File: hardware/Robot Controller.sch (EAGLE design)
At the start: 17 parts

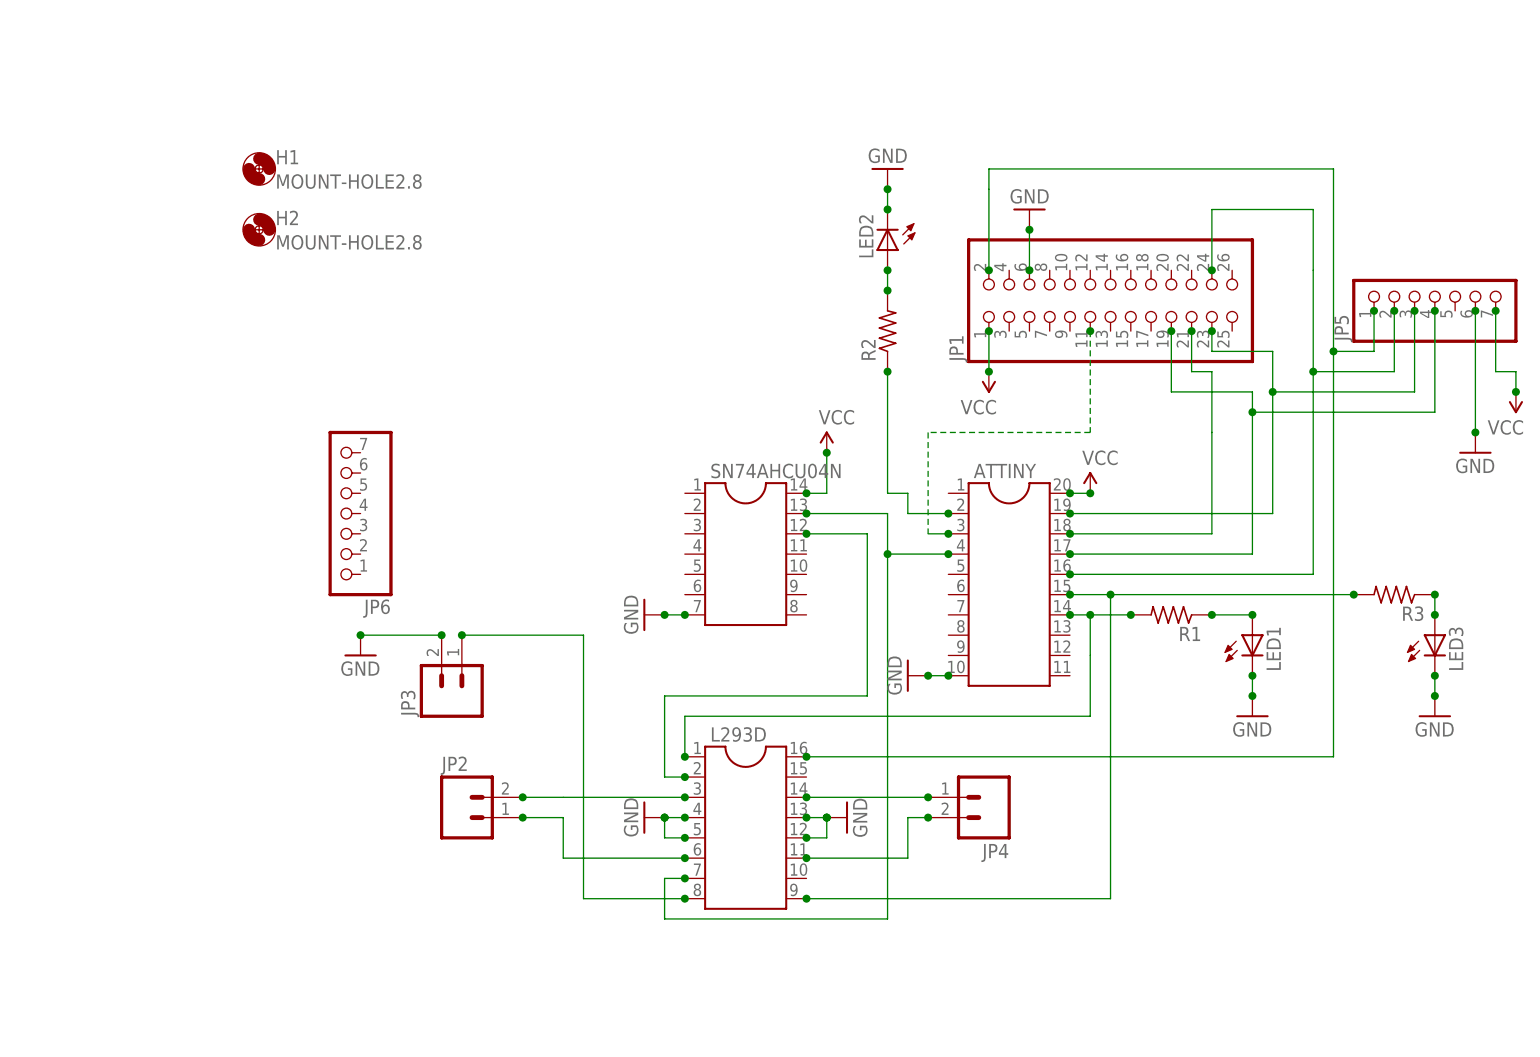
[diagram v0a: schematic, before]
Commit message: WIP dev board
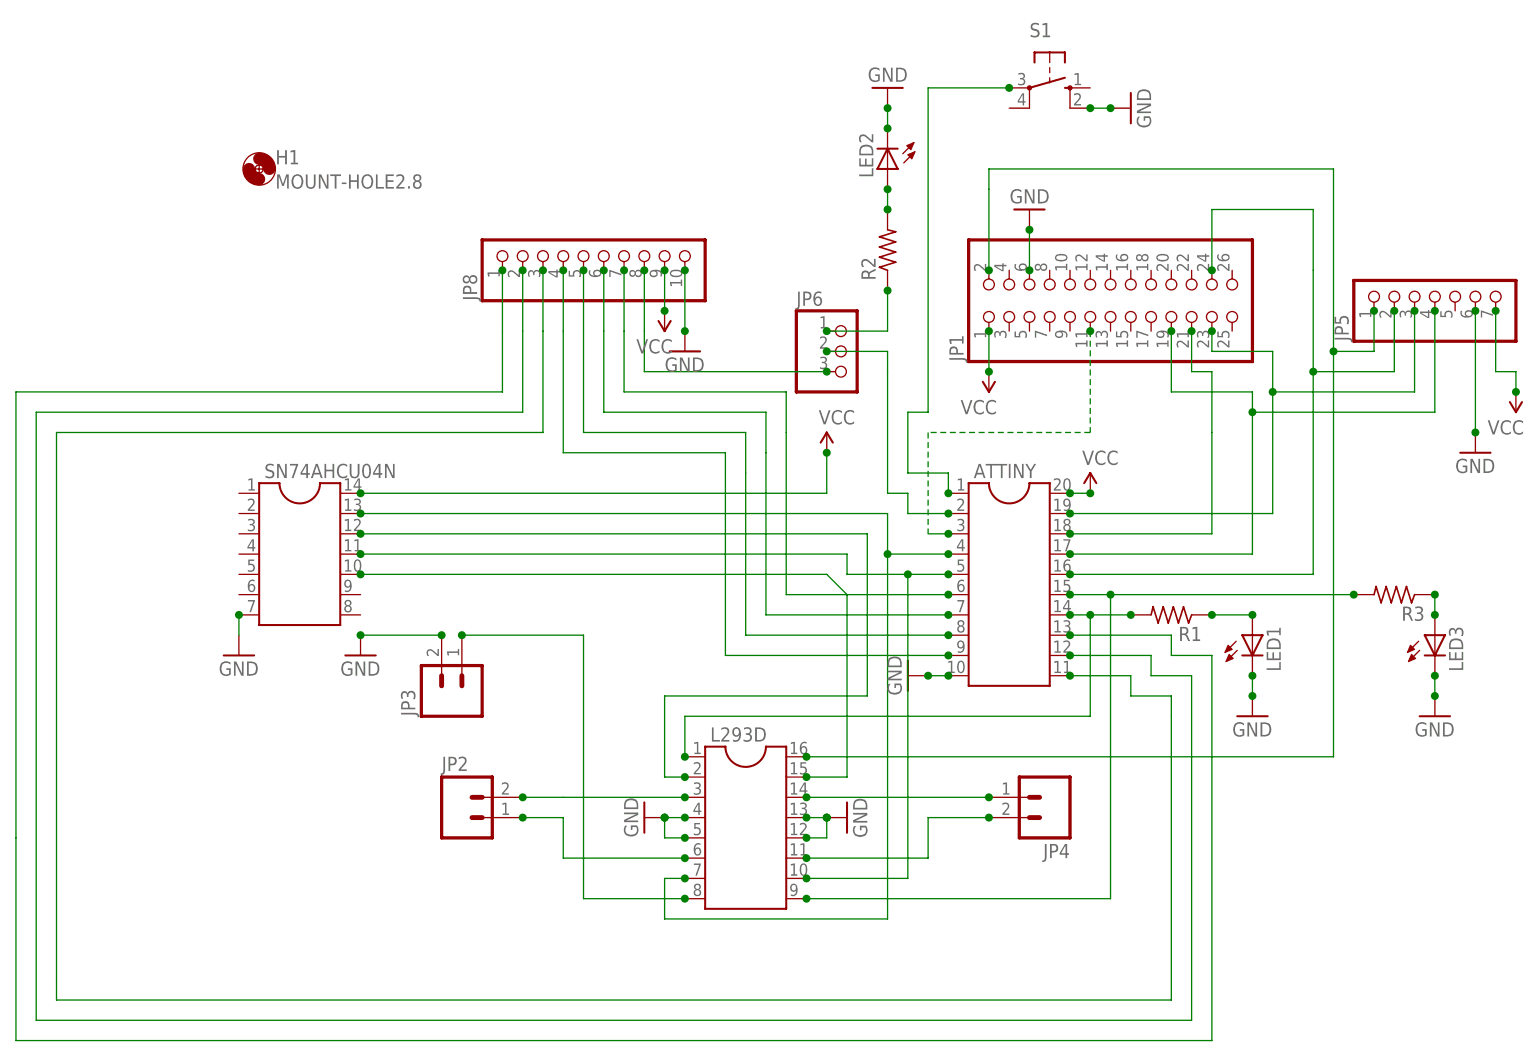
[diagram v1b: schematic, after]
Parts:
- removed H2: MOUNT-HOLE2.8, holes:MOUNT-HOLE2.8
- added JP8: (no value), pinhead:PINHD-1X10
- added S1: (no value), switch-omron:10-XX
- JP6: device pinhead:PINHD-1X7 -> pinhead:PINHD-1X3
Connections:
- new net N$20: ATTINY.5, L293D.10, SN74AHCU04N.11
- new net N$21: JP6.1, R2.1
- new net N$22: L293D.15, SN74AHCU04N.10
- new net N$23: JP6.3, JP8.8
- new net N$24: ATTINY.6, JP8.7
- new net N$25: ATTINY.7, JP8.6
- new net N$26: ATTINY.8, JP8.5
- new net N$27: ATTINY.9, JP8.4
- new net N$28: ATTINY.13, JP8.1
- new net N$29: ATTINY.12, JP8.2
- new net N$30: ATTINY.11, JP8.3
- new net N$31: ATTINY.1, S1.P
- net GND: now also JP8.10, S1.S1
- net N$16: now also JP6.2; no longer R2.1
- net VCC: now also JP8.9
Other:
- moved on the sheet: JP4, LED2, R2, SN74AHCU04N
